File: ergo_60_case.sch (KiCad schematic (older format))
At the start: 24 parts, among them SW1 SW_Push, U1 PRTR5V0U2X, U2 OLED_SSD1306, U3 AT90USB1286-AU, U4 AVR-ISP, Y1 16MHz

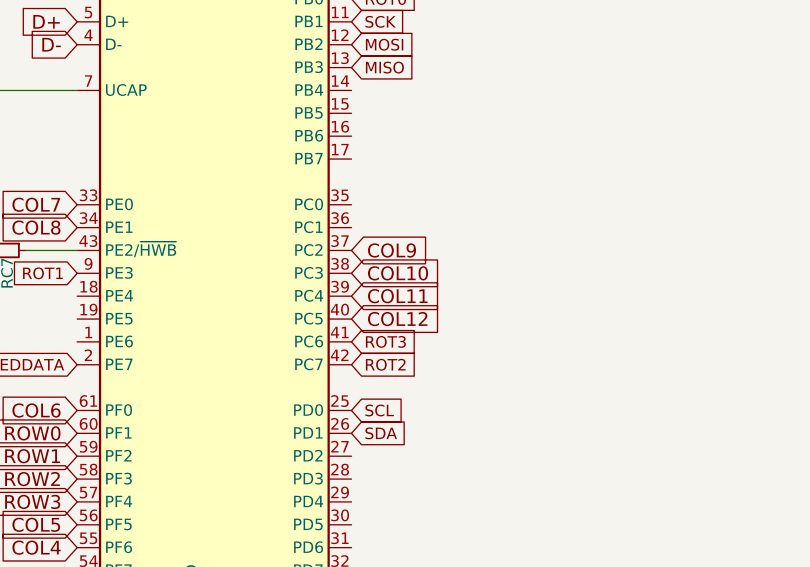
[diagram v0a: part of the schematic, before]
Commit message: progress
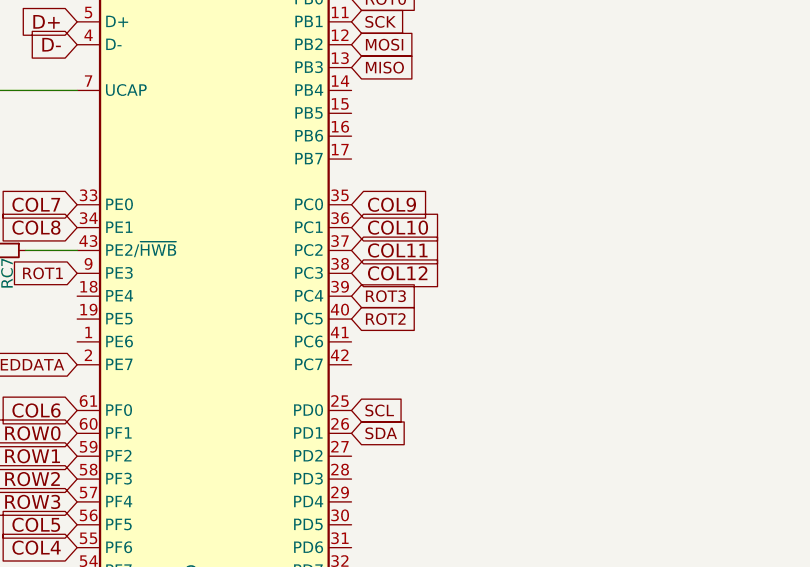
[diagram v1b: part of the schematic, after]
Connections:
- net COL10: now also U3.36 (PC1); no longer U3.38 (PC3)
- net COL11: now also U3.37 (PC2); no longer U3.39 (PC4)
- net COL12: now also U3.38 (PC3); no longer U3.40 (PC5)
- net COL9: now also U3.35 (PC0); no longer U3.37 (PC2)
- net ROT2: now also U3.40 (PC5); no longer U3.42 (PC7)
- net ROT3: now also U3.39 (PC4); no longer U3.41 (PC6)
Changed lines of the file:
@@
 Text GLabel 4675 5275 0    60   Input ~ 0
 COL8
+Text GLabel 5875 5175 2    60   Input ~ 0
+COL9
+Text GLabel 5875 5275 2    60   Input ~ 0
+COL10
 Text GLabel 5875 5375 2    60   Input ~ 0
-COL9
+COL11
 Text GLabel 5875 5475 2    60   Input ~ 0
-COL10
-Text GLabel 5875 5575 2    60   Input ~ 0
-COL11
-Text GLabel 5875 5675 2    60   Input ~ 0
 COL12
 Text GLabel 5875 3675 2    60   Input ~ 0
@@
 Text GLabel 4675 5475 0    50   Input ~ 0
 ROT1
-Text GLabel 5875 5875 2    50   Input ~ 0
+Text GLabel 5875 5675 2    50   Input ~ 0
 ROT2
-Text GLabel 5875 5775 2    50   Input ~ 0
+Text GLabel 5875 5575 2    50   Input ~ 0
 ROT3
 Text GLabel 4675 5875 0    50   Input ~ 0
